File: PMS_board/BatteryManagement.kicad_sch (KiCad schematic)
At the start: 39 parts, among them IC1 L9962-TR, SW1 PWR_SW

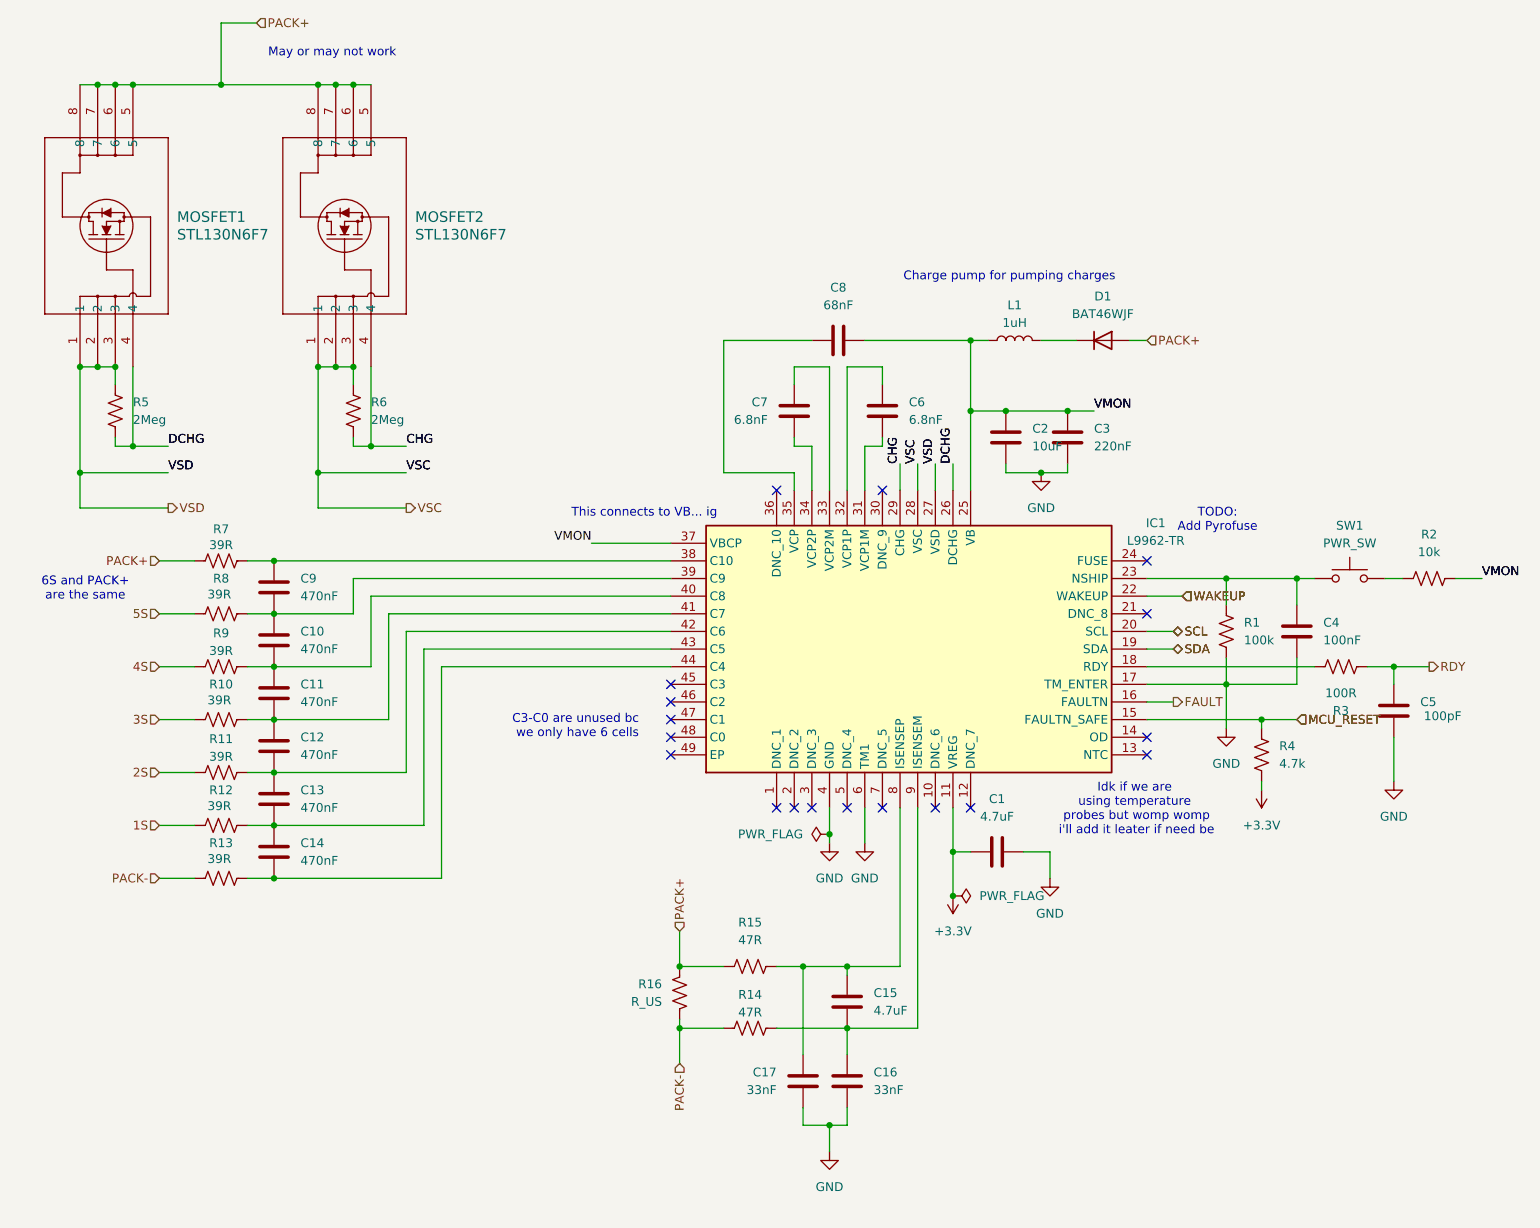
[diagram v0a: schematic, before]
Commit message: Restored to stable commit
Idk wtf i'm doing
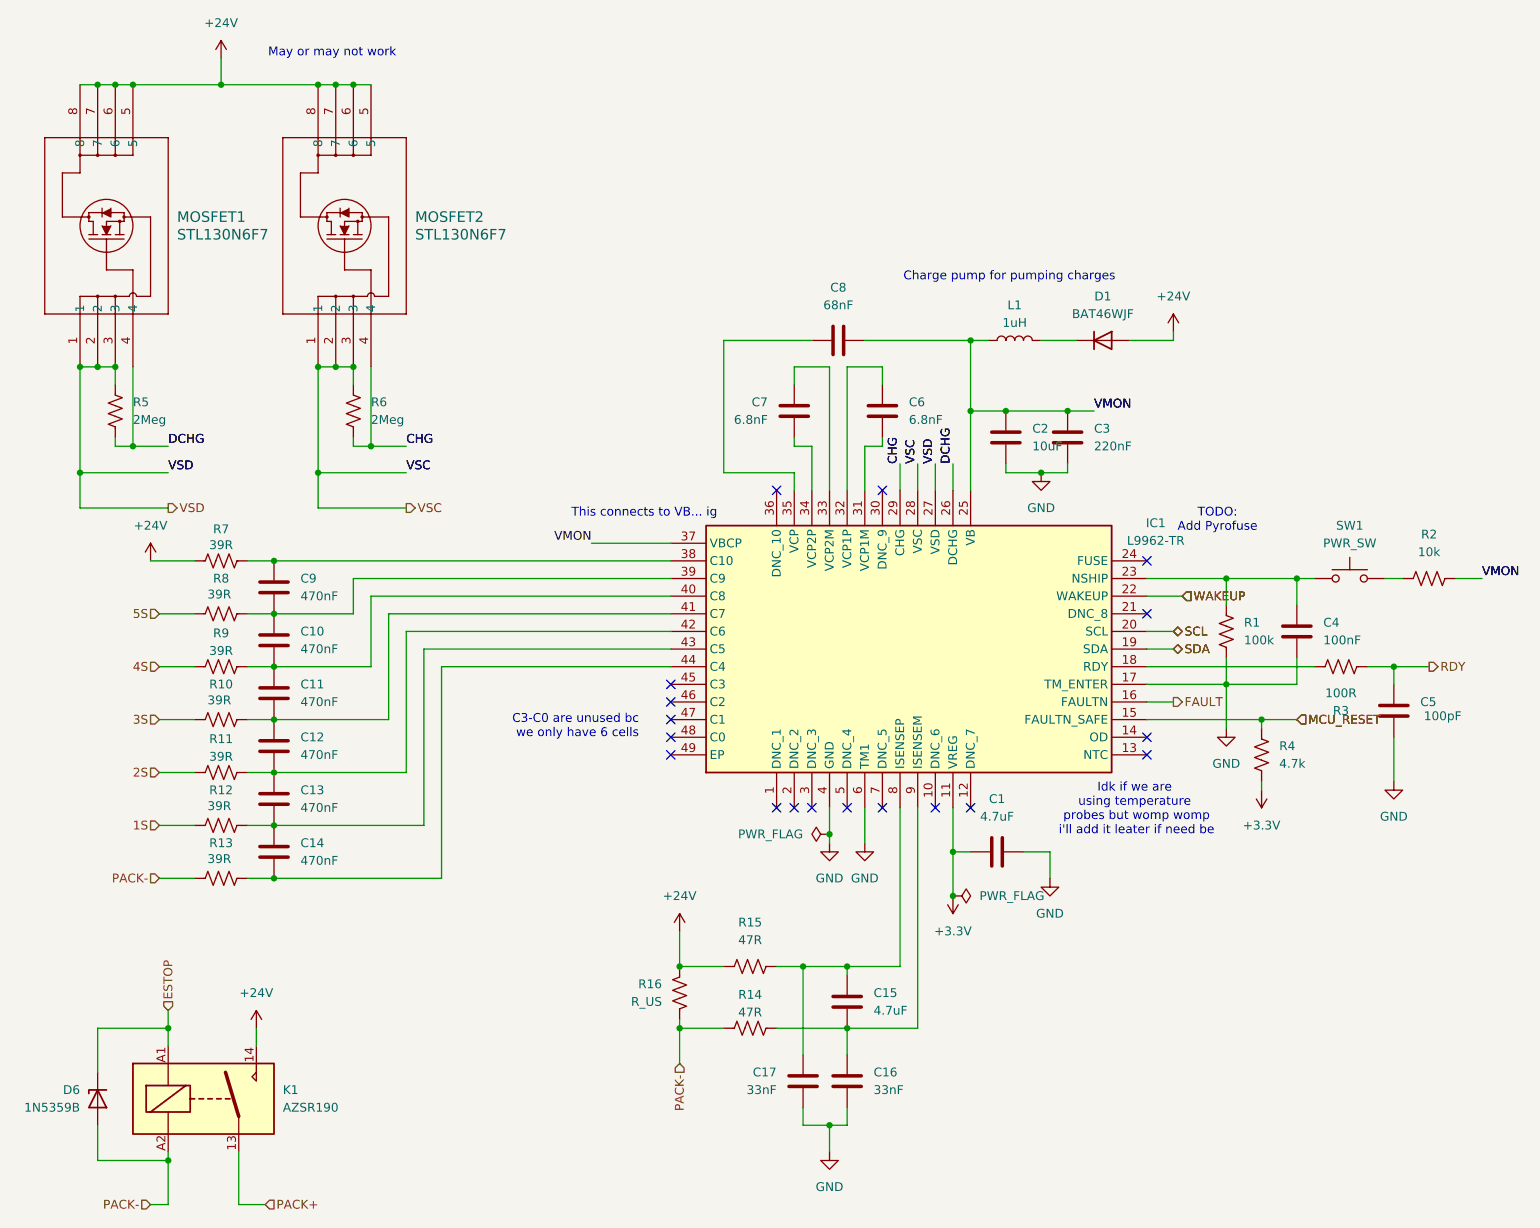
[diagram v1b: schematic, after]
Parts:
- added D6: 1N5359B, Diode_THT:D_DO-201_P15.24mm_Horizontal, symbol Diode:1N53xxB
- added K1: AZSR190, Relay_THT:Relay_SPST-NO_Fujitsu_FTR-LYAA005x_FormA_Vertical, symbol Relay:Relay_SPST-NO
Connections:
- net PACK+: now also K1.13; no longer D1.2 (A), MOSFET1.5, MOSFET1.6, MOSFET1.7, MOSFET1.8, MOSFET2.5, MOSFET2.6, MOSFET2.7, MOSFET2.8, R15.1, R16.1, R7.1
- net PACK-: now also D6.2 (A), K1.A2
- new net +24V: D1.2 (A), K1.14, MOSFET1.5, MOSFET1.6, MOSFET1.7, MOSFET1.8, MOSFET2.5, MOSFET2.6, MOSFET2.7, MOSFET2.8, R15.1, R16.1, R7.1
- new net ESTOP: D6.1 (K), K1.A1
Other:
- note removed: "6S and PACK+ are the same"

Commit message: Revert "Merge branch '2027_Rev1' of https://github.com/MissouriMRDT/PowerManagement_Hardware into 2027_Rev1"
This reverts commit 58e8d8a37d7e6e053a99adaceb0a0b64a7e4d5ac, reversing
changes made to 2dbcd4446407a5b00bde621a86c6c0759956a2a3.
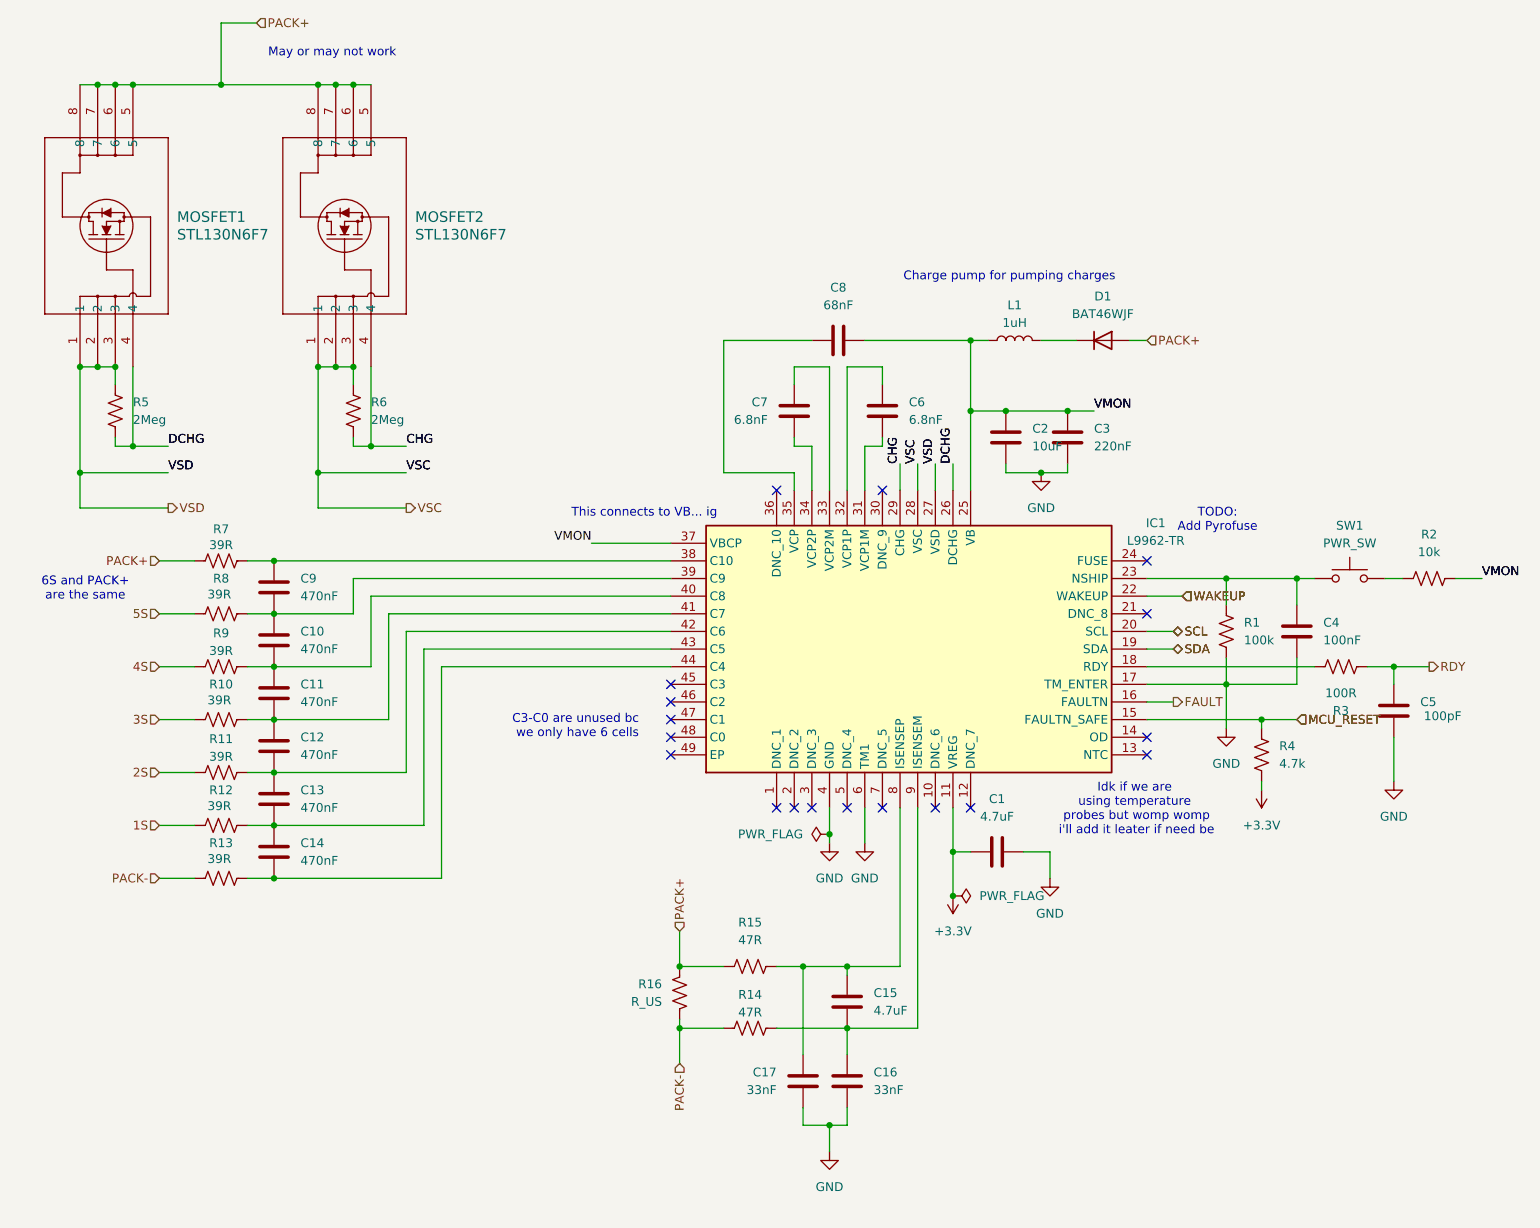
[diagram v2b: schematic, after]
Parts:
- removed D6: 1N5359B, Diode_THT:D_DO-201_P15.24mm_Horizontal, symbol Diode:1N53xxB
- removed K1: AZSR190, Relay_THT:Relay_SPST-NO_Fujitsu_FTR-LYAA005x_FormA_Vertical, symbol Relay:Relay_SPST-NO
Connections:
- net +24V is gone; now on net PACK+: D1.2 (A), MOSFET1.5, MOSFET1.6, MOSFET1.7, MOSFET1.8, MOSFET2.5, MOSFET2.6, MOSFET2.7, MOSFET2.8, R15.1, R16.1, R7.1
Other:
- note added: "6S and PACK+ are the same"
